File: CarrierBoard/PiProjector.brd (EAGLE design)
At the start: 86.4 x 54.6 mm, 74 parts, among them P8 PINHEAD2X23, P9 PINHEAD2X23, Q2 BSS84, X1 24MHz, X2 12Mhz

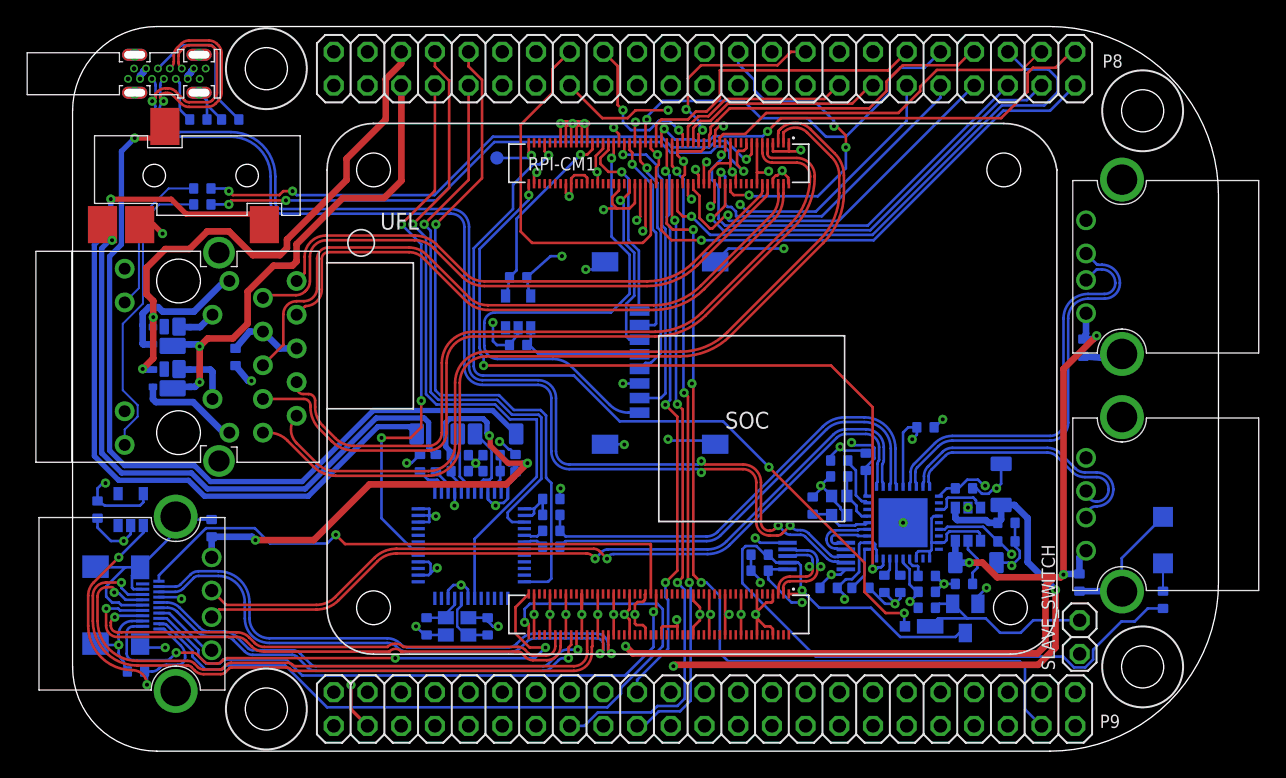
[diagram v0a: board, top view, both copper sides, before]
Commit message: minor fixes
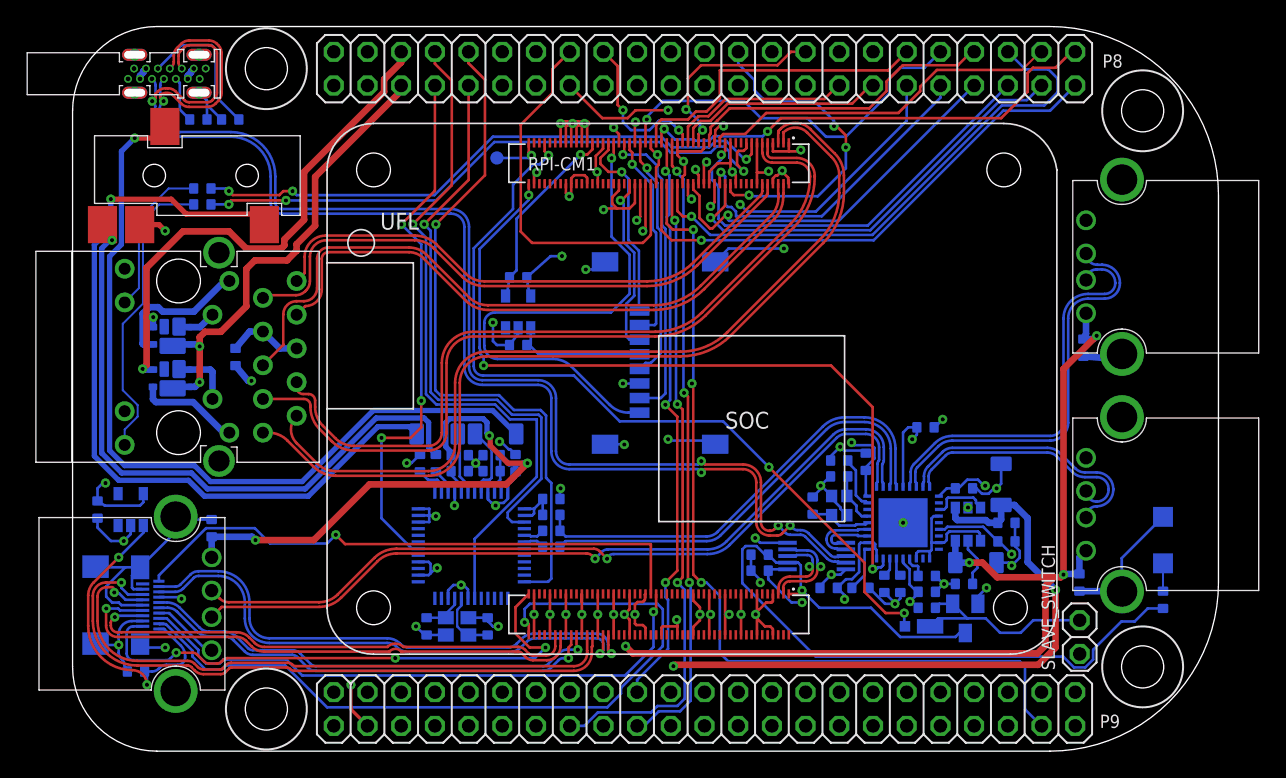
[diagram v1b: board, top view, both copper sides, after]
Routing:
- net POE+: track 34.2 -> 32.6 mm
- net GND: track 231.5 -> 230.0 mm
